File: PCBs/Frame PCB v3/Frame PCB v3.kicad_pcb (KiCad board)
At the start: 2 copper layers, 78 x 40.6 mm, 16 parts, among them J1 Nichrome 1, J2 Nichrome 2, J3 Battery in, J6 Switch, q1 Voltage regulator

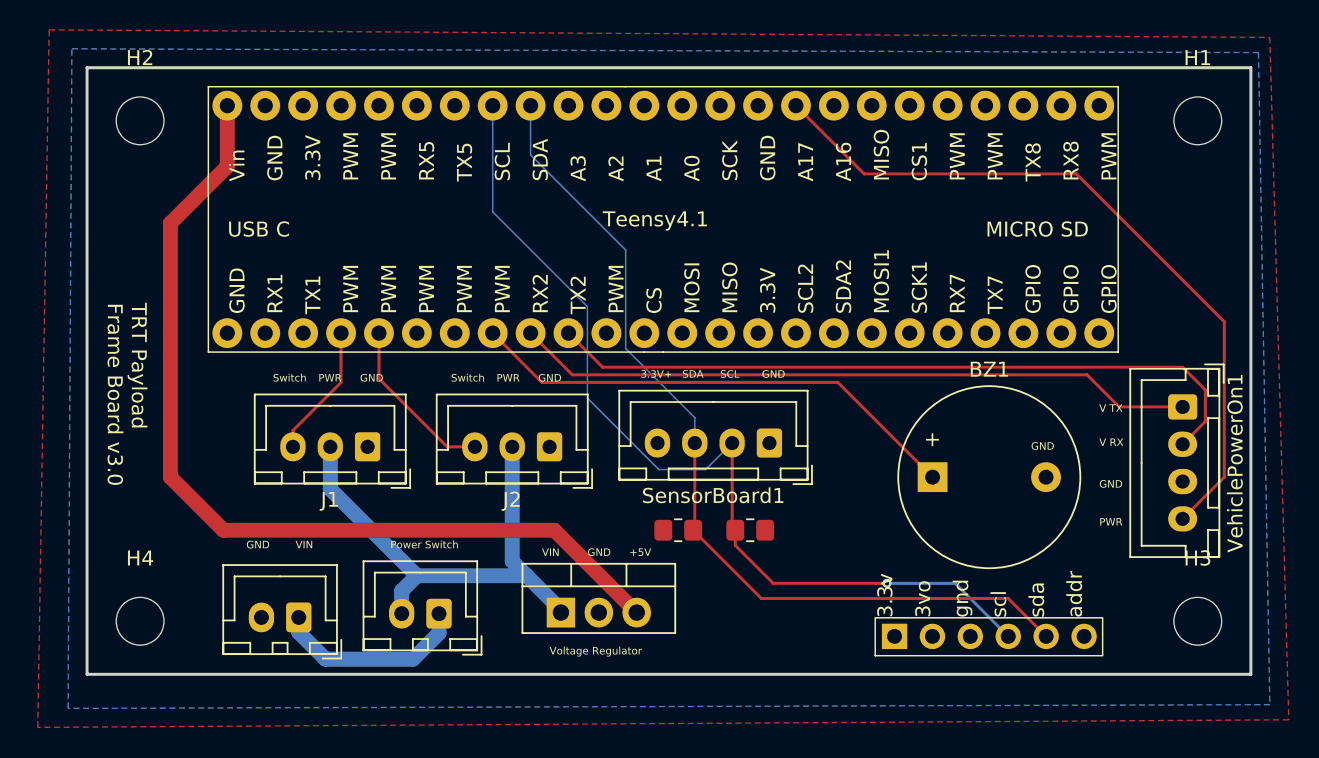
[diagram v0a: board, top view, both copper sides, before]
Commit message: updated PCBS
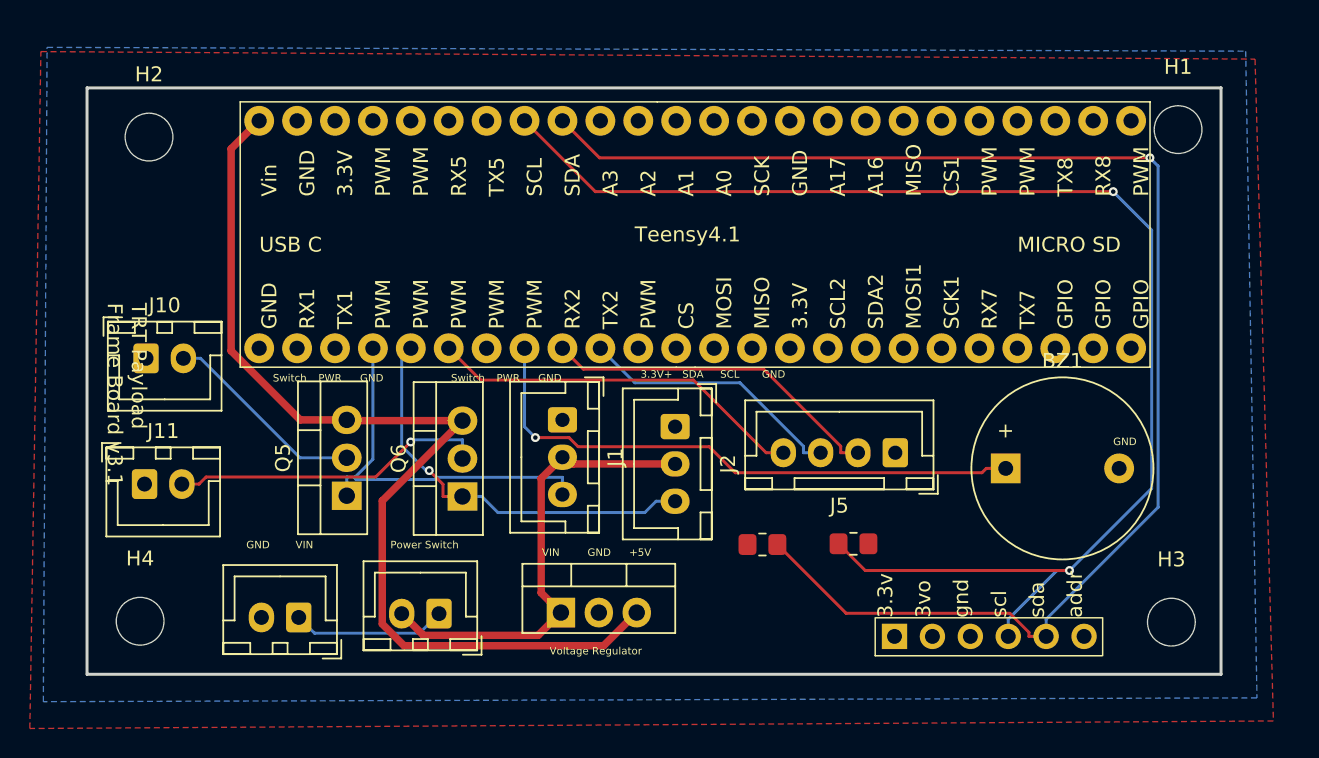
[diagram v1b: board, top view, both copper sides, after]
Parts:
- removed SensorBoard1, VehiclePowerOn1: I2C Connector, Connector_JST:JST_XH_B4B-XH-A_1x04_P2.50mm_Vertical
- added J10: Nichrome, Connector_JST:JST_XH_B2B-XH-A_1x02_P2.50mm_Vertical, F.Cu at (121.3, 73.8)
- added J11: Nichrome, Connector_JST:JST_XH_B2B-XH-A_1x02_P2.50mm_Vertical, F.Cu at (121.2, 82.2)
- added J5: BayConnector, Connector_JST:JST_XH_B4B-XH-A_1x04_P2.50mm_Vertical, F.Cu at (171.5, 80.2)
- added Q5: Nichrome, Package_TO_SOT_THT:TO-220-3_Vertical, F.Cu at (134.8, 83.0)
- added Q6: Nichrome, Package_TO_SOT_THT:TO-220-3_Vertical, F.Cu at (142.5, 83.1)
- moved J1 13.2 mm to (149.2, 78.0), turned to -90 degrees
- moved J2 8.52 mm to (156.8, 78.4), turned to -90 degrees
- moved R2 6.98 mm to (168.7, 86.2)
- moved R1 5.72 mm to (162.6, 86.3)
- moved BZ1 4.94 mm to (178.9, 81.2)
- moved Teensy4.1 2.36 mm to (158.1, 65.5)
- moved H3 1.77 mm to (190.0, 91.5)
- moved H1 1.45 mm to (190.4, 58.5)
- moved H2 1.24 mm to (121.5, 59.0)
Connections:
- Teensy4.1 pad 32: VehicleSwitch -> unconnected-(Teensy4.1-A17-Pad32)
- Teensy4.1 pad 5: unconnected-(Teensy4.1-PWM-Pad5) -> VehicleOn
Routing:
- net VehicleSwitch: track 49.1 -> 0.00 mm
- net SDA: track 59.7 -> 96.5 mm, vias 0 -> 1
- net VehicleRX: track 48.5 -> 17.9 mm
- net SCL: track 62.4 -> 93.0 mm, vias 1 -> 2
- net VehicleOn: track 0.00 -> 25.3 mm
- net VehicleTX: track 45.7 -> 23.0 mm
- net Net-(J11-Pin_2): track 0.00 -> 21.3 mm, vias 0 -> 1
- net Nichrome1: track 8.95 -> 26.2 mm
- net Nichrome2: track 11.4 -> 27.8 mm, vias 0 -> 1
- net Net-(J10-Pin_2): track 0.00 -> 13.7 mm
- net +5V: track 61.5 -> 68.0 mm
- net BuzzerPin: track 33.5 -> 38.9 mm, vias 0 -> 1
- net Net-(J3-Pin_1): track 13.2 -> 10.4 mm
- net +9V: track 33.8 -> 31.2 mm
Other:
- board size 78 x 40.6 mm -> 76 x 39.3 mm
- board text added: "TRT Payload Frame Board v3.1"
- board text removed: "TRT Payload Frame Board v3.0"
- board text removed: "V RX"
- board text removed: "V TX"
